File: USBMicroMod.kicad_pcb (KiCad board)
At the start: 2 copper layers, 59 x 25.5 mm, 9 parts, among them J1 MICROMOD-2222-C, J2 USB_A, U1 PLUG, U2 PLUG

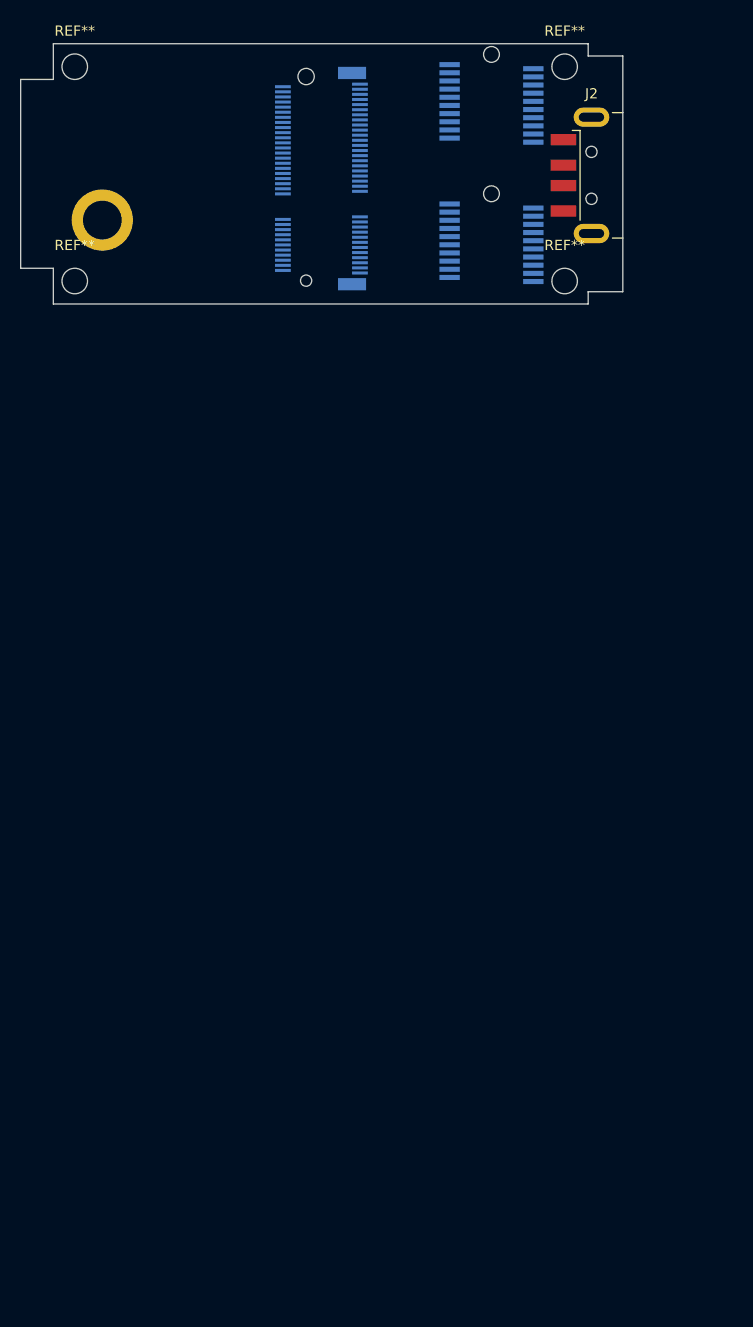
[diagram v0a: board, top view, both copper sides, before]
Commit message: Final v1
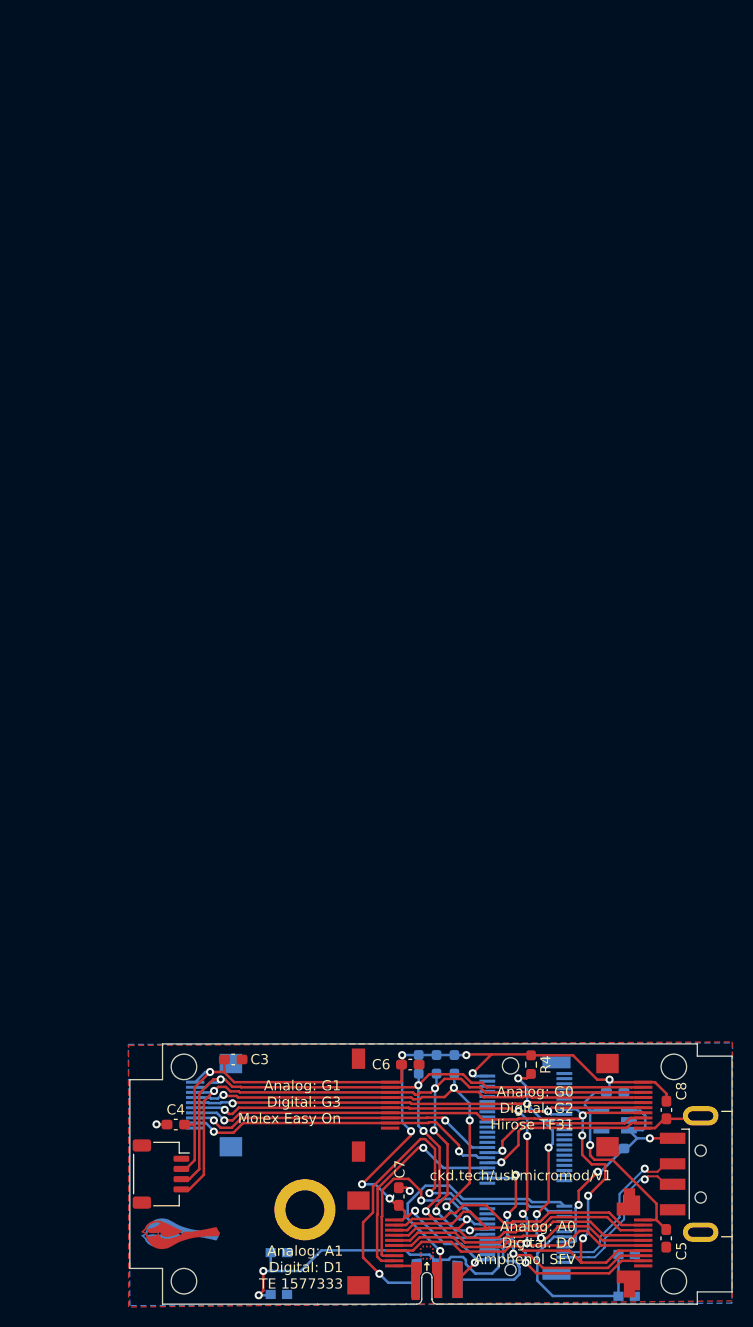
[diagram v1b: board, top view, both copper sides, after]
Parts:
- removed U2: PLUG, PLUG:PLUG
- added C1: 1uF, Capacitor_SMD:C_0603_1608Metric_Pad1.08x0.95mm_HandSolder, B.Cu at (163.2, 84.8)
- added C2: 1uF, Capacitor_SMD:C_0603_1608Metric_Pad1.08x0.95mm_HandSolder, B.Cu at (163.2, 79.2)
- added C3: 1uF, Capacitor_SMD:C_0603_1608Metric_Pad1.08x0.95mm_HandSolder, F.Cu at (125.8, 76.0)
- added C4: 1uF, Capacitor_SMD:C_0603_1608Metric_Pad1.08x0.95mm_HandSolder, F.Cu at (120.2, 82.4)
- added C5: 1uF, Capacitor_SMD:C_0603_1608Metric_Pad1.08x0.95mm_HandSolder, F.Cu at (168.2, 93.5)
- added C6: 1uF, Capacitor_SMD:C_0603_1608Metric_Pad1.08x0.95mm_HandSolder, F.Cu at (143.2, 76.5)
- added C7: 1uF, Capacitor_SMD:C_0603_1608Metric_Pad1.08x0.95mm_HandSolder, F.Cu at (142.1, 89.5)
- added C8: 1uF, Capacitor_SMD:C_0603_1608Metric_Pad1.08x0.95mm_HandSolder, F.Cu at (168.3, 81.0)
- added G***: Chickadee 3mm, chickadee:chickadee_3mm_fcu, B.Cu at (120.6, 93.0)
- added G***: Chickadee 3mm, chickadee:chickadee_3mm_fcu, F.Cu at (120.6, 93.2)
- added J3: DebugEdge_02x03, Connector_DebugEdge:DebugEdge_2x03_Target, F.Cu at (145.8, 100.0)
- added J4: Conn_01x10, 10posFPC:Hirose-TF31, F.Cu at (165.1, 80.5)
- added J5: Conn_01x10, 10posFPC:Amphenol-SFV, F.Cu at (165.1, 94.0)
- added J6: Conn_01x10, 10posFPC:Molex-Easy-On, F.Cu at (140.3, 80.5)
- added J7: Conn_01x10, 10posFPC:TE-1775333, F.Cu at (140.7, 94.0)
- added J8: Conn_01x10, 10posFPC:Hirose-TF31, B.Cu at (123.0, 80.5)
- added J9: Conn_01x04_Male, Connector_JST:JST_SH_SM04B-SRSS-TB_1x04-1MP_P1.00mm_Horizontal, F.Cu at (118.8, 87.2)
- added R1: 2.2k, Resistor_SMD:R_0603_1608Metric_Pad0.98x0.95mm_HandSolder, B.Cu at (144.0, 76.5)
- added R2: 2.2k, Resistor_SMD:R_0603_1608Metric_Pad0.98x0.95mm_HandSolder, B.Cu at (145.8, 76.5)
- added R3: 2.2k, Resistor_SMD:R_0603_1608Metric_Pad0.98x0.95mm_HandSolder, B.Cu at (147.5, 76.5)
- added R4: 100k, Resistor_SMD:R_0603_1608Metric_Pad0.98x0.95mm_HandSolder, F.Cu at (155.0, 76.5)
- added SW1: SW_Push, Button_Switch_SMD:SW_Push_1P1T_NO_CK_KMR2, B.Cu at (130.3, 97.0)
- added SW2: SW_Push, Button_Switch_SMD:SW_Push_1P1T_NO_CK_KMR2, B.Cu at (164.4, 97.2)
- U1: value PLUG -> AP2112K-3.3; footprint PLUG:PLUG -> Package_TO_SOT_SMD:SOT-23-5_HandSoldering
- moved U1 100.4 mm to (163.2, 82.0), turned to 180 degrees
- moved J1 99.0 mm to (153.0, 86.7)
- moved H5 99.0 mm to (132.8, 90.8)
- moved REF** 98.6 mm to (169.0, 97.8)
- moved REF** 98.6 mm to (121.0, 97.8)
- moved REF** 98.6 mm to (169.0, 76.8)
- moved REF** 98.6 mm to (121.0, 76.8)
- moved J2 98.4 mm to (178.5, 87.2)
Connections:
- net /BATT renamed Net-(J1-Pad49)
- net /CHIP_SELECT renamed Net-(J1-Pad70)
- J1 pad 11: Net-(J1-Pad11) -> /~BOOT
- J1 pad 12: /I2C_SDA -> /SDA
- J1 pad 14: /I2C_SCL -> /SCL
- J1 pad 16: /I2C_~INT -> /INT
- J1 pad 18: Net-(J1-Pad18) -> /D1
- J1 pad 40: Net-(J1-Pad40) -> /A2
- J1 pad 42: Net-(J1-Pad42) -> /A3
- J1 pad 44: Net-(J1-Pad44) -> /D2
- J1 pad 46: Net-(J1-Pad46) -> /D3
- J1 pad 57: Net-(J1-Pad57) -> /SCK
- J1 pad 59: Net-(J1-Pad59) -> /MOSI
- J1 pad 6: Net-(J1-Pad6) -> /~RESET
- J1 pad 60: /SCK -> Net-(J1-Pad60)
- J1 pad 61: Net-(J1-Pad61) -> /MISO
- J1 pad 62: /MOSI -> Net-(J1-Pad62)
- J1 pad 64: /MISO -> Net-(J1-Pad64)
- J1 pad 8: Net-(J1-Pad8) -> /SWO
- U1 pad 1: Net-(U1-Pad1) -> VBUS
- U1 pad 2: Net-(U1-Pad2) -> GND
- U1 pad 3: Net-(U1-Pad3) -> VBUS
- U1 pad 5: Net-(U1-Pad5) -> +3V3
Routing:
- net +3V3: track 0.00 -> 127.9 mm, vias 0 -> 11
- net /SDA: track 0.00 -> 108.0 mm, vias 0 -> 4
- net /SCL: track 0.00 -> 106.2 mm, vias 0 -> 5
- net /INT: track 0.00 -> 92.1 mm, vias 0 -> 5
- net /SCK: track 0.00 -> 92.1 mm, vias 0 -> 6
- net /MISO: track 0.00 -> 90.8 mm, vias 0 -> 5
- net /MOSI: track 0.00 -> 86.7 mm, vias 0 -> 6
- net /SWCLK: track 0.00 -> 40.5 mm, vias 0 -> 2
- net /~RESET: track 0.00 -> 36.2 mm, vias 0 -> 2
- net /A3: track 0.00 -> 31.3 mm, vias 0 -> 2
- net /D3: track 0.00 -> 30.7 mm, vias 0 -> 2
- net /A0: track 0.00 -> 25.1 mm, vias 0 -> 3
- net /SWDIO: track 0.00 -> 24.6 mm, vias 0 -> 1
- net VBUS: track 0.00 -> 23.3 mm, vias 0 -> 3
- net /A1: track 0.00 -> 21.8 mm, vias 0 -> 1
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- added copper zone on B.Cu, net GND
- added copper zone on F.Cu, net GND
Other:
- outline, holes or cut-outs redrawn
- board text added: "Analog: A0 Digital: D0 Amphenol SFV"
- board text added: "Analog: A1 Digital: D1 TE 1577333"
- board text added: "Analog: G0 Digital: G2 Hirose TF31"
- board text added: "Analog: G1 Digital: G3 Hirose TF31"
- board text added: "Analog: G1 Digital: G3 Molex Easy On"
- board text added: "BOOT"
- board text added: "ckd.tech/usbmicromod/v1"
- board text added: "~RESET"
